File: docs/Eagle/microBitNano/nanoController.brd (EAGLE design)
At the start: 63.6 x 80 mm, 12 parts, among them J2 MTXNRX, J3 IR RX, J4 IR TX, J8 MRXNTX

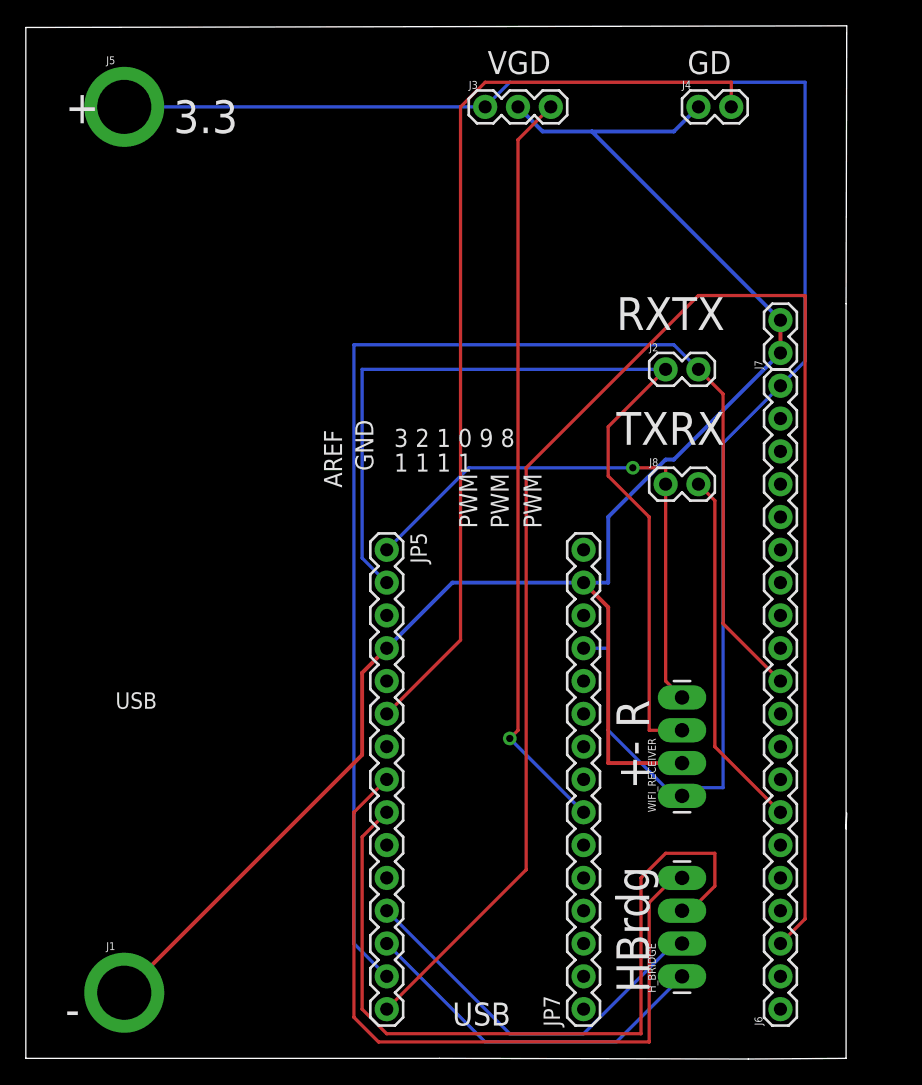
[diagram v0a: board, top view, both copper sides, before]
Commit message: crossover
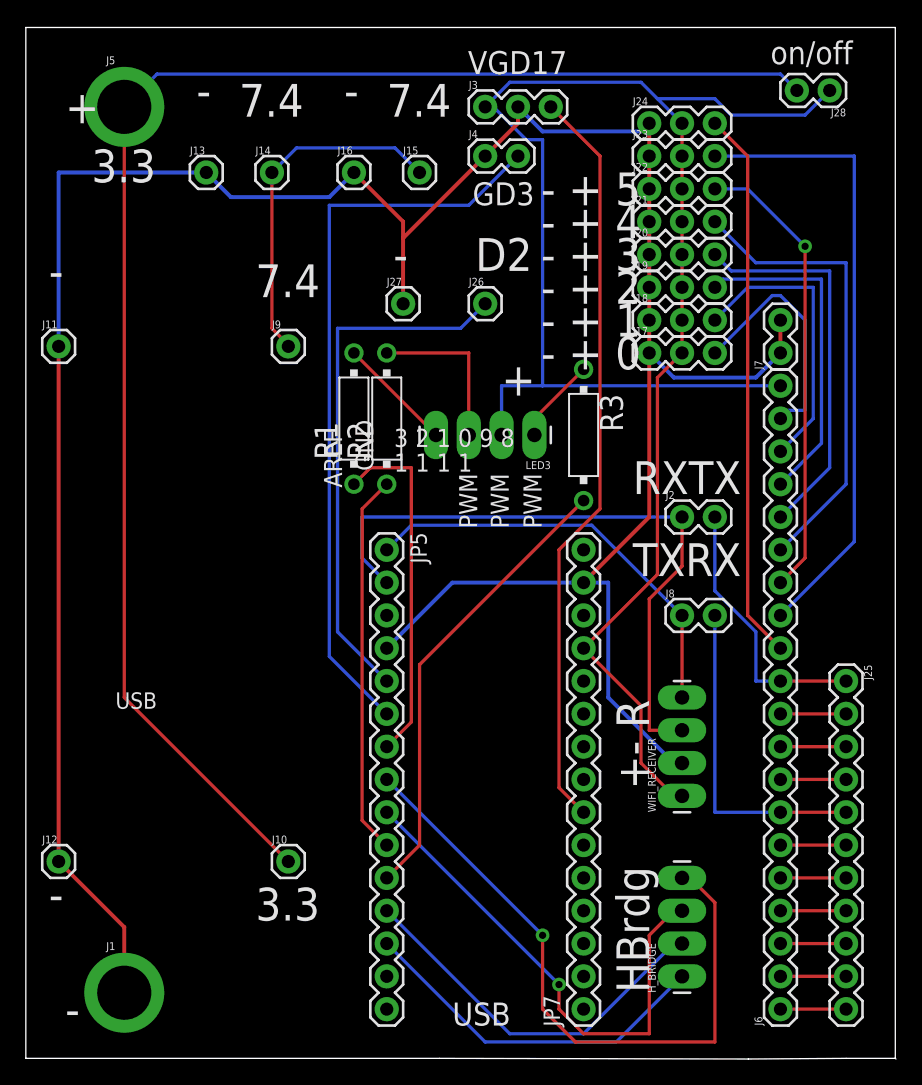
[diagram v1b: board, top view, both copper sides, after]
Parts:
- added J10, J11, J12, J13, J14, J15, J16, J26, J27, J9: (no value), SparkFun-Connectors:1X01
- added J17, J18, J19, J20, J21, J22, J23, J24: IR RX, SparkFun-Connectors:1X03
- added J25: (no value), SparkFun-Connectors:1X11
- added J28: MTXNRX, SparkFun-Connectors:1X02
- added LED3: (no value), SparkFun-Connectors:1X04_LONGPADS
- added R1, R2, R3: (no value), resistor-power:HPS58
- moved J4 16.9 mm to (35.6, 69.8)
- moved J2 11.5 mm to (50.8, 41.9)
- moved J8 10.2 mm to (50.8, 34.3)
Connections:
- new net 3.3V: J10.1, J28.2, J5.P$1
- new net 7.4V: J14.1, J15.1, J9.1
- new net D11: JP5.14
- new net D12: JP5.15
- new net N$1: LED3.4, R1.2
- new net N$2: LED3.3, R2.2
- new net N$3: LED3.1, R3.1
- net D2: now also J26.1
- net D4: now also R1.1
- net D7: now also R2.1
- net D8: now also R3.2
- net GND: now also J11.1, J12.1, J13.1, J16.1, J17.1, J18.1, J19.1, J20.1, J21.1, J22.1, J23.1, J24.1, J27.1
- net M0: now also J17.3
- net M1: now also J18.3
- net M10: now also J25.3
- net M11: now also J25.4
- net M12: now also J25.5
- net M13: now also J25.6
- net M14: now also J25.7
- net M15: now also J25.8
- net M16: now also J25.9; no longer JP5.15
- net M19: now also J25.10
- net M2: now also J19.3
- net M20: now also J25.11
- net M3: now also J20.3
- net M4: now also J21.3
- net M5: now also J22.3
- net M6: now also J23.3
- net M7: now also J24.3
- net M8: now also J25.1; no longer JP5.14
- net M9: now also J25.2
- net VCC: now also J17.2, J18.2, J19.2, J20.2, J21.2, J22.2, J23.2, J24.2, J28.1, LED3.2; no longer J5.P$1
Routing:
- net M16: track 124.4 -> 5.08 mm
- net 3.3V: track 0.00 -> 117.3 mm
- net M8: track 104.2 -> 21.0 mm
- net GND: track 137.2 -> 214.7 mm
- net M6: track 0.00 -> 48.7 mm
- net M7: track 0.00 -> 42.7 mm
- net D2: track 0.00 -> 41.1 mm
- net M4: track 0.00 -> 35.8 mm
- net M5: track 0.00 -> 35.7 mm, vias 0 -> 1
- net D8: track 0.00 -> 35.5 mm
- net M3: track 0.00 -> 30.0 mm
- net D7: track 0.00 -> 29.5 mm
- net D4: track 0.00 -> 27.4 mm
- net 7.4V: track 0.00 -> 27.0 mm
- net M2: track 0.00 -> 25.7 mm
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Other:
- board size 63.6 x 80 mm -> 67.4 x 79.9 mm
- board text added: "- + 0"
- board text added: "- + 1"
- board text added: "- + 2"
- board text added: "- + 3"
- board text added: "- + 4"
- board text added: "- + 5"
- board text added: "7.4"
- board text added: "D2"
- board text added: "GD3"
- board text added: "VGD17"
- board text added: "on/off"
- board text removed: "GD"
- board text removed: "VGD"
